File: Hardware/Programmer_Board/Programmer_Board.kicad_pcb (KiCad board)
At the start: 4 copper layers, 49.1 x 15.5 mm, 58 parts, among them J101 IDC Connector, J102 PicoBlade, J103 USB_C_USB2.0, U1 TPD4E02B04, U102 TPS7A20L_3V3, U103 USBLC6-2SC6, U201 FT2232HQ, U202 93LC56B, Y201 16MHz

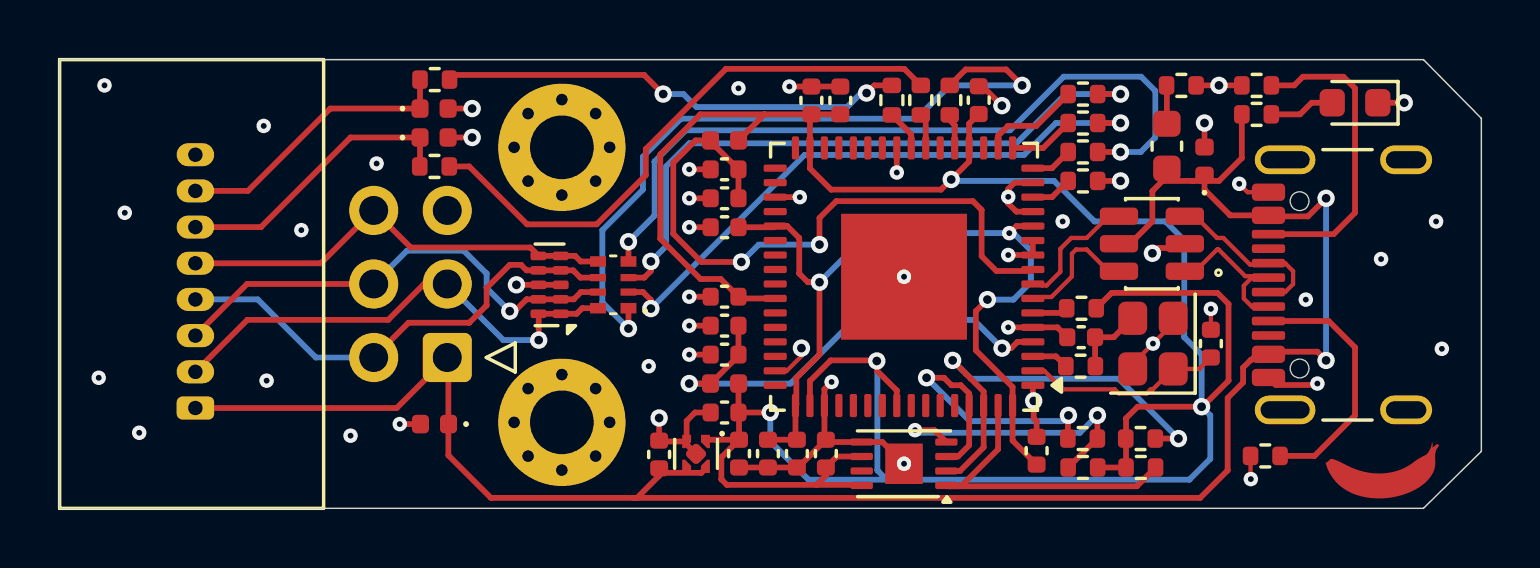
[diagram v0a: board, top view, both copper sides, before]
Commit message: Updated documentation and finished first iteration of PCB rework based on manufacturer feedback.
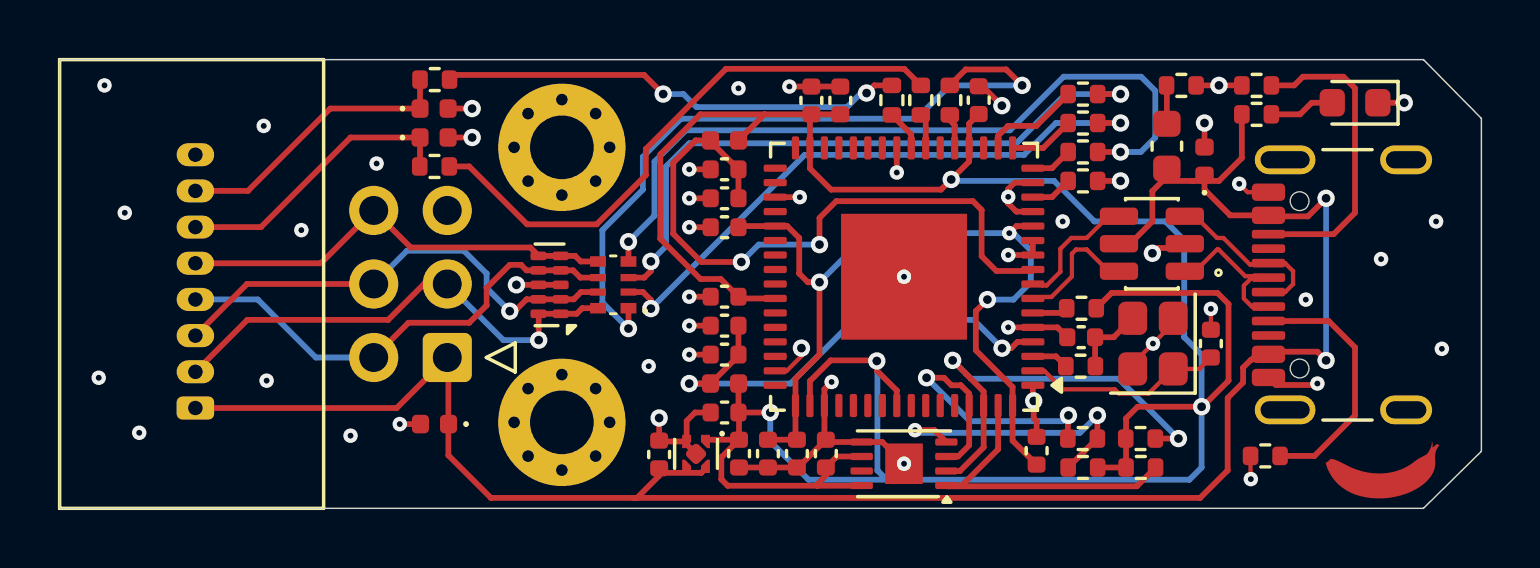
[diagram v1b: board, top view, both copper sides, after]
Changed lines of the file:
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@@
 		)
 		(embedded_fonts no)
-		(model "${KICAD9_3DMODEL_DIR}/Diode_SMD.3dshapes/D_0402_1005Metric.step"
+		(model "${KICAD9_3DMODEL_DIR}/Diode_SMD.3dshapes/D_0603_1608Metric.step"
 			(offset
 				(xyz 0 0 0)
 			)
 			(scale
-				(xyz 1 1 1)
+				(xyz 0.7 0.7 0.7)
 			)
 			(rotate
-				(xyz 0 0 0)
+				(xyz -0 -0 -0)
 			)
 		)
@@
 		)
 		(embedded_fonts no)
-		(model "${KICAD9_3DMODEL_DIR}/Diode_SMD.3dshapes/D_0402_1005Metric.step"
+		(model "${KICAD9_3DMODEL_DIR}/Diode_SMD.3dshapes/D_0603_1608Metric.step"
 			(offset
 				(xyz 0 0 0)
 			)
 			(scale
-				(xyz 1 1 1)
+				(xyz 0.7 0.7 0.7)
 			)
 			(rotate
-				(xyz 0 0 0)
+				(xyz -0 -0 -0)
 			)
 		)
@@
 		)
 		(embedded_fonts no)
-		(model "${KICAD9_3DMODEL_DIR}/Package_SON.3dshapes/Texas_X2SON-4_1x1mm_P0.65mm.step"
+		(model "C:/Users/varsa/Desktop/School/5_semester/BachelorProject/VoxLink/Hardware/libraries/3D/TPS7A20L33PDQNR.stp"
 			(offset
 				(xyz 0 0 0)
@@
 			)
 			(rotate
-				(xyz 0 0 0)
+				(xyz -90 -0 -0)
 			)
 		)
@@
 	)
 	(segment
+		(start 157.07 110.83)
+		(end 157.1 110.8)
+		(width 0.2)
+		(layer "F.Cu")
+		(net 3)
+	)
+	(segment
 		(start 155.57 108.06)
 		(end 155.57 107.213798)
@@
 	)
 	(segment
-		(start 166.49 110.2)
-		(end 166.49 108.5)
+		(start 155.8 110.8)
+		(end 155.83 110.83)
 		(width 0.2)
 		(layer "F.Cu")
@@
 	)
 	(segment
-		(start 152.509 110.609)
-		(end 152.7 110.8)
+		(start 166.49 110.2)
+		(end 166.49 108.5)
 		(width 0.2)
 		(layer "F.Cu")
@@
 	)
 	(segment
+		(start 152.509 109.851)
+		(end 152.509 110.609)
+		(width 0.2)
+		(layer "F.Cu")
+		(net 3)
+	)
+	(segment
 		(start 161.07 99.16)
 		(end 161.07 98.32)
@@
 	)
 	(segment
-		(start 153.12 109.24)
-		(end 152.509 109.851)
+		(start 156.62 98)
+		(end 155.62 98)
 		(width 0.2)
 		(layer "F.Cu")
@@
 	)
 	(segment
-		(start 156.62 98)
-		(end 155.62 98)
+		(start 152.509 110.609)
+		(end 152.73 110.83)
 		(width 0.2)
 		(layer "F.Cu")
@@
 	)
 	(segment
-		(start 152.7 110.8)
-		(end 155.8 110.8)
+		(start 166.89 108.1)
+		(end 169.1 108.1)
 		(width 0.2)
 		(layer "F.Cu")
@@
 	)
 	(segment
-		(start 166.89 108.1)
-		(end 169.1 108.1)
+		(start 152.73 110.83)
+		(end 155.83 110.83)
 		(width 0.2)
 		(layer "F.Cu")
@@
 	)
 	(segment
+		(start 155.83 110.83)
+		(end 157.07 110.83)
+		(width 0.2)
+		(layer "F.Cu")
+		(net 3)
+	)
+	(segment
 		(start 155.57 99.87)
 		(end 155.57 99.16)
@@
 	)
 	(segment
+		(start 153.12 109.24)
+		(end 152.509 109.851)
+		(width 0.2)
+		(layer "F.Cu")
+		(net 3)
+	)
+	(segment
 		(start 169.1329 108.1)
 		(end 170.031 107.2019)
@@
 	)
 	(segment
-		(start 155.8 110.8)
-		(end 157.1 110.8)
-		(width 0.2)
-		(layer "F.Cu")
-		(net 3)
-	)
-	(segment
 		(start 153.1 98.9)
 		(end 154 98)
@@
 		(net 3)
 	)
-	(segment
-		(start 152.509 109.851)
-		(end 152.509 110.609)
-		(width 0.2)
-		(layer "F.Cu")
-		(net 3)
-	)
 	(via
 		(at 169.1 108.1)
@@
 	)
 	(segment
-		(start 169.4 108.4)
-		(end 169.1 108.1)
-		(width 0.2)
-		(layer "B.Cu")
-		(net 3)
-	)
-	(segment
 		(start 158.221 110.621)
 		(end 168.679 110.621)
@@
 	)
 	(segment
-		(start 168.679 110.621)
-		(end 169.4 109.9)
+		(start 160.5 100.3)
+		(end 160.45 100.25)
 		(width 0.2)
 		(layer "B.Cu")
@@
 	)
 	(segment
-		(start 160.5 100.3)
-		(end 160.45 100.25)
+		(start 168.679 110.621)
+		(end 169.1 110.2)
 		(width 0.2)
 		(layer "B.Cu")
@@
 	)
 	(segment
-		(start 169.4 109.9)
-		(end 169.4 108.4)
+		(start 169.1 110.2)
+		(end 169.1 108.1)
 		(width 0.2)
 		(layer "B.Cu")
@@
 	)
 	(segment
-		(start 167.415 107.5)
-		(end 167.340804 107.5)
-		(width 0.15)
-		(layer "F.Cu")
-		(net 6)
-	)
-	(segment
-		(start 167.340804 107.5)
-		(end 167.194804 107.646)
-		(width 0.15)
-		(layer "F.Cu")
-		(net 6)
-	)
-	(segment
-		(start 167.194804 107.646)
-		(end 166.245196 107.646)
+		(start 164.305016 107.5)
+		(end 166.099196 107.5)
 		(width 0.15)
 		(layer "F.Cu")
@@
 	)
 	(segment
-		(start 166.099196 107.5)
-		(end 164.305016 107.5)
+		(start 167.269 107.646)
+		(end 168.12 106.795)
 		(width 0.15)
 		(layer "F.Cu")
@@
 	)
 	(segment
-		(start 168.12 106.795)
-		(end 167.415 107.5)
+		(start 163.665016 106.86)
+		(end 164.305016 107.5)
 		(width 0.15)
 		(layer "F.Cu")
@@
 	)
 	(segment
-		(start 166.245196 107.646)
-		(end 166.099196 107.5)
+		(start 163.27 106.86)
+		(end 163.665016 106.86)
 		(width 0.15)
 		(layer "F.Cu")
@@
 	)
 	(segment
-		(start 163.665016 106.86)
-		(end 163.27 106.86)
+		(start 166.245196 107.646)
+		(end 167.269 107.646)
 		(width 0.15)
 		(layer "F.Cu")
@@
 	)
 	(segment
-		(start 164.305016 107.5)
-		(end 163.665016 106.86)
+		(start 166.099196 107.5)
+		(end 166.245196 107.646)
 		(width 0.15)
 		(layer "F.Cu")
@@
 	)
 	(segment
-		(start 155.9 106.3)
-		(end 155.1 107.1)
-		(width 0.2)
-		(layer "F.Cu")
-		(net 8)
-	)
-	(segment
 		(start 161.7 104.4)
 		(end 161.3 104.8)
@@
 	)
 	(segment
-		(start 155.1 107.1)
-		(end 155.1 108.03)
+		(start 155.07 108.06)
+		(end 155.07 109.19)
 		(width 0.2)
 		(layer "F.Cu")
@@
 	)
 	(segment
-		(start 155.07 108.06)
-		(end 155.07 109.19)
+		(start 153.14 101.86)
+		(end 154.37 101.86)
 		(width 0.2)
 		(layer "F.Cu")
@@
 	)
 	(segment
+		(start 155.9 106.3)
+		(end 155.07 107.13)
+		(width 0.2)
+		(layer "F.Cu")
+		(net 8)
+	)
+	(segment
 		(start 162.57 108.06)
 		(end 162.57 109.27)
@@
 	)
 	(segment
+		(start 153.1 101.9)
+		(end 153.14 101.86)
+		(width 0.2)
+		(layer "F.Cu")
+		(net 8)
+	)
+	(segment
 		(start 155.2 102.274202)
 		(end 155.2 103.5)
@@
 	)
 	(segment
-		(start 153.1 101.9)
-		(end 154.33 101.9)
-		(width 0.2)
-		(layer "F.Cu")
-		(net 8)
-	)
-	(segment
-		(start 154.33 101.9)
-		(end 154.37 101.86)
-		(width 0.2)
-		(layer "F.Cu")
-		(net 8)
-	)
-	(segment
 		(start 162.57 107.419943)
 		(end 162.57 108.06)
@@
 	)
 	(segment
-		(start 155.1 108.03)
+		(start 155.07 107.13)
 		(end 155.07 108.06)
 		(width 0.2)
